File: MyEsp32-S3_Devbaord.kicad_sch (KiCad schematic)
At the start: 31 parts, among them J1 USB_C_Receptacle_USB2.0_16P, J2 Conn_01x22, J3 Conn_01x22, SW1 ~{RESET}, SW2 ~{BOOT}, U1 ESP32-S3-MINI-1, U2 MPU-9250, U3 AMS1117-3.3, U4 NTC0805J10K, U5 USBLC6-2SC6, U6 Square_Small

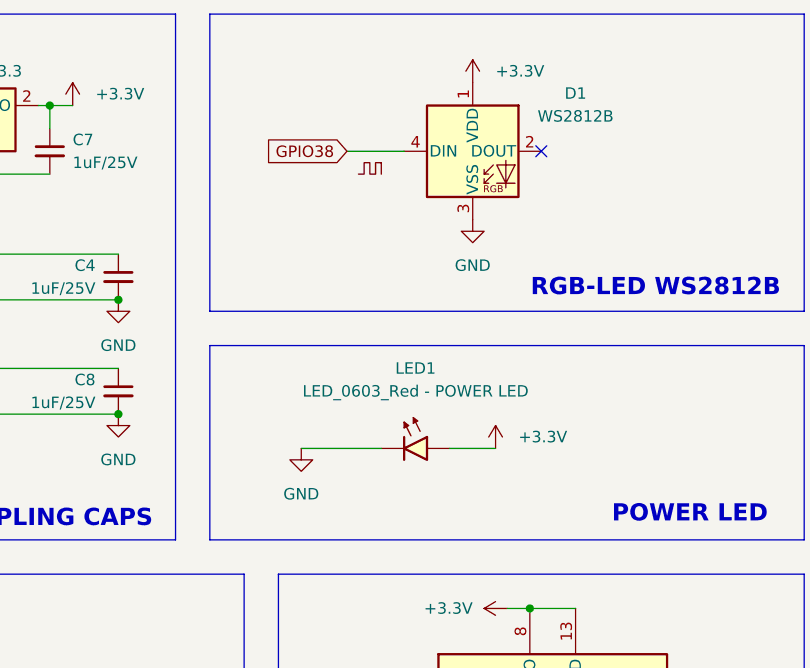
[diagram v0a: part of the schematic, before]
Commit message: Add files via upload
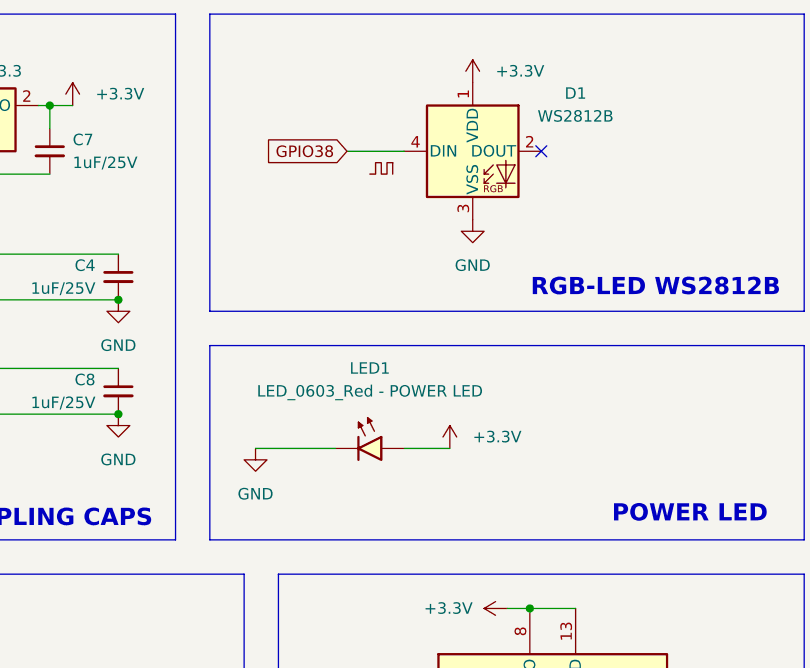
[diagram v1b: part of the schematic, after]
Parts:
- R3: footprint 4ms_Resistor:R_0603 -> Resistor_SMD:R_0603_1608Metric
- U1: footprint easyeda2kicad:WIRELM-SMD_ESP32-S3-WROOM-1 -> PCM_Espressif:ESP32-S2-MINI-1
- U4: footprint easyeda2kicad:R0805 -> EasyEDA2Kicad:R0805
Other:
- moved on the sheet: LED1
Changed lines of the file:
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@@
 	(wire
 		(pts
-			(xy 140.97 63.5) (xy 149.86 63.5)
+			(xy 135.89 63.5) (xy 144.78 63.5)
 		)
 		(stroke
@@
 	(wire
 		(pts
-			(xy 157.48 63.5) (xy 162.56 63.5)
+			(xy 152.4 63.5) (xy 157.48 63.5)
 		)
 		(stroke
@@
 			)
 		)
-		(property "Footprint" "easyeda2kicad:WIRELM-SMD_ESP32-S3-WROOM-1"
+		(property "Footprint" "PCM_Espressif:ESP32-S2-MINI-1"
 			(at 73.66 185.42 0)
 			(effects
@@
 	(symbol
 		(lib_id "power:+3.3V")
-		(at 162.56 63.5 0)
+		(at 157.48 63.5 0)
 		(unit 1)
 		(exclude_from_sim no)
@@
 		(fields_autoplaced yes)
 		(property "Reference" "#PWR023"
-			(at 162.56 67.31 0)
+			(at 157.48 67.31 0)
 			(effects
 				(font
@@
 		)
 		(property "Value" "+3.3V"
-			(at 165.1 62.2299 0)
+			(at 160.02 62.2299 0)
 			(effects
 				(font
@@
 		)
 		(property "Footprint" ""
-			(at 162.56 63.5 0)
+			(at 157.48 63.5 0)
 			(effects
 				(font
@@
 		)
 		(property "Datasheet" ""
-			(at 162.56 63.5 0)
+			(at 157.48 63.5 0)
 			(effects
 				(font
@@
 		)
 		(property "Description" "Power symbol creates a global label with name \"+3.3V\""
-			(at 162.56 63.5 0)
+			(at 157.48 63.5 0)
 			(effects
 				(font
@@
 			)
 		)
-		(property "Sim.Enable" "0"
-			(at 251.46 156.21 0)
-			(effects
-				(font
-					(size 1.27 1.27)
-				)
-				(hide yes)
-			)
-		)
 		(instances
 			(project ""
@@
 	(symbol
 		(lib_id "PCM_LED_AKL:LED_0603_Red")
-		(at 153.67 63.5 0)
+		(at 148.59 63.5 0)
 		(mirror y)
 		(unit 1)
@@
 		(fields_autoplaced yes)
 		(property "Reference" "LED1"
-			(at 153.67 54.61 0)
+			(at 148.59 54.61 0)
 			(effects
 				(font
@@
 		)
 		(property "Value" "LED_0603_Red - POWER LED"
-			(at 153.67 57.15 0)
+			(at 148.59 57.15 0)
 			(effects
 				(font
@@
 		)
 		(property "Footprint" "PCM_LED_SMD_AKL:LED_0603_1608Metric"
-			(at 153.67 63.5 0)
+			(at 148.59 63.5 0)
 			(effects
 				(font
@@
 		)
 		(property "Datasheet" "~"
-			(at 153.67 63.5 0)
+			(at 148.59 63.5 0)
 			(effects
 				(font
@@
 		)
 		(property "Description" "Red SMD LED, 0603, Alternate KiCad Library"
-			(at 153.67 63.5 0)
+			(at 148.59 63.5 0)
 			(effects
 				(font
@@
 	(symbol
 		(lib_id "PCM_Graphics_AKL:Square_Small")
-		(at 148.59 33.02 0)
+		(at 149.86 33.02 0)
 		(unit 1)
 		(exclude_from_sim no)
@@
 		(fields_autoplaced yes)
 		(property "Reference" "U6"
-			(at 148.59 33.02 0)
+			(at 149.86 33.02 0)
 			(effects
 				(font
@@
 		)
 		(property "Value" "Square_Small"
-			(at 148.59 33.02 0)
+			(at 149.86 33.02 0)
 			(effects
 				(font
@@
 		)
 		(property "Footprint" ""
-			(at 148.59 33.02 0)
+			(at 149.86 33.02 0)
 			(effects
 				(font
@@
 		)
 		(property "Datasheet" ""
-			(at 148.59 33.02 0)
+			(at 149.86 33.02 0)
 			(effects
 				(font
@@
 		)
 		(property "Description" "Small Square-Wave Symbol"
-			(at 148.59 33.02 0)
+			(at 149.86 33.02 0)
 			(effects
 				(font
@@
 			)
 		)
-		(property "Sim.Enable" "0"
-			(at 238.76 156.21 0)
-			(effects
-				(font
-					(size 1.27 1.27)
-				)
-				(hide yes)
-			)
-		)
 		(instances
 			(project ""
@@
 			)
 		)
-		(property "Footprint" "4ms_Resistor:R_0603"
+		(property "Footprint" "Resistor_SMD:R_0603_1608Metric"
 			(at 181.61 154.94 0)
 			(effects
@@
 	(symbol
 		(lib_id "power:GND")
-		(at 140.97 63.5 0)
+		(at 135.89 63.5 0)
 		(unit 1)
 		(exclude_from_sim no)
@@
 		(fields_autoplaced yes)
 		(property "Reference" "#PWR022"
-			(at 140.97 69.85 0)
+			(at 135.89 69.85 0)
 			(effects
 				(font
@@
 		)
 		(property "Value" "GND"
-			(at 140.97 68.58 0)
+			(at 135.89 68.58 0)
 			(effects
 				(font
@@
 		)
 		(property "Footprint" ""
-			(at 140.97 63.5 0)
+			(at 135.89 63.5 0)
 			(effects
 				(font
@@
 		)
 		(property "Datasheet" ""
-			(at 140.97 63.5 0)
+			(at 135.89 63.5 0)
 			(effects
 				(font
@@
 		)
 		(property "Description" "Power symbol creates a global label with name \"GND\" , ground"
-			(at 140.97 63.5 0)
+			(at 135.89 63.5 0)
 			(effects
 				(font
@@
 			)
 		)
-		(property "Footprint" "easyeda2kicad:R0805"
+		(property "Footprint" "EasyEDA2Kicad:R0805"
 			(at 153.67 160.02 0)
 			(effects
@@
 			(at 264.16 156.21 0)
 			(effects
-				(font
-					(size 1.27 1.27)
-				)
-				(hide yes)
-			)
-		)
-		(property "Sim.Enable" "0"
-			(at 264.16 156.21 0)
-			(effects
